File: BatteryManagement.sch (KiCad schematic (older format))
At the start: 1 part

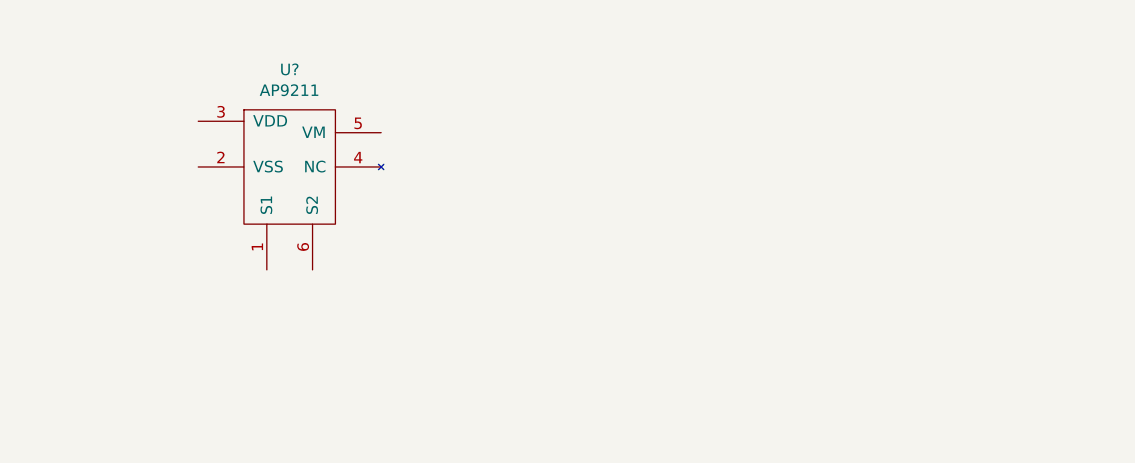
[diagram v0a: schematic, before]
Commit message: Battery work, need to get on to connectors.
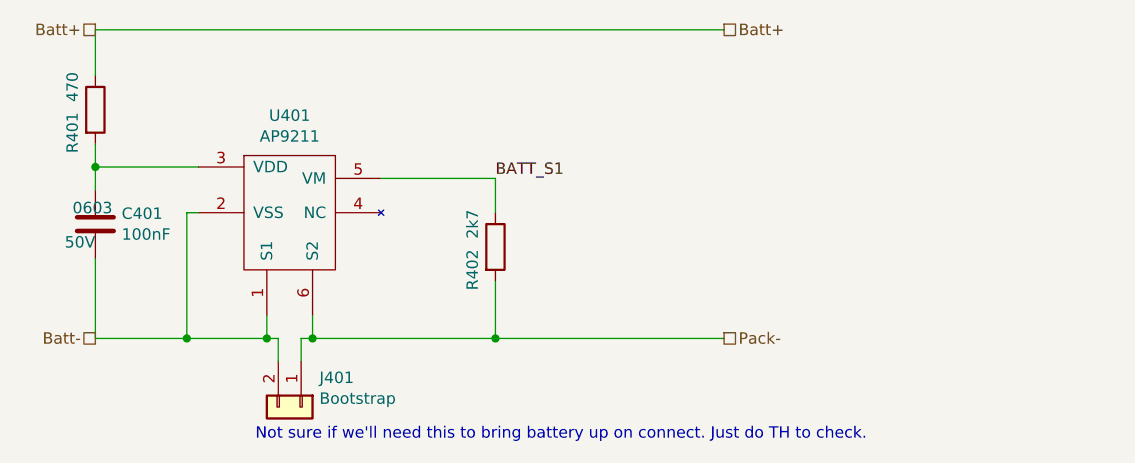
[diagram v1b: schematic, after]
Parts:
- added C401: 100nF, Capacitors_SMD:C_0603, symbol Device:C
- added J401: Bootstrap, Pin_Headers:Pin_Header_Straight_1x02_Pitch2.54mm, symbol Connector_Generic:Conn_01x02
- added R401: 470, Resistor_SMD:R_0603_1608Metric_Pad1.05x0.95mm_HandSolder, symbol Device:R
- added R402: 2k7, Resistor_SMD:R_0603_1608Metric_Pad1.05x0.95mm_HandSolder, symbol Device:R
- gave numbers to parts that had none: 1
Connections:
- net Batt-: now reaches U401.1 (S1)
- net Batt-: now also U401.2 (VSS), C401.2, J401.2 (Pin_2)
- net at U401.3 (VDD): now also C401.1, R401.2
- net BATT_S1: now reaches U401.5 (VM)
- net BATT_S1: now also R402.1
- net Pack-: now reaches U401.6 (S2)
- net Pack-: now also J401.1 (Pin_1), R402.2
- new net Batt+: R401.1
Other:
- note added: "Not sure if we'll need this to bring battery up on connect. Just do TH to check."
- moved on the sheet: U401
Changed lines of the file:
@@
 L dingo-hat:AP9211 U?
 U 1 1 5DC173E3
-P 5550 2800
+P 5550 3000
 AR Path="/5DA95EB0/5DAAD200/5DC173E3" Ref="U?"  Part="1"
-AR Path="/5DC297AB/5DC173E3" Ref="U?"  Part="1"
-F 0 "U?" H 5550 3225 50  0000 C CNN
-F 1 "AP9211" H 5550 3134 50  0000 C CNN
-F 2 "" H 5550 2650 50  0001 C CNN
-F 3 "https://www.diodes.com/assets/Datasheets/AP9211.pdf" H 5550 2650 50  0001 C CNN
-	1    5550 2800
+AR Path="/5DC297AB/5DC173E3" Ref="U401"  Part="1"
+F 0 "U401" H 5550 3425 50  0000 C CNN
+F 1 "AP9211" H 5550 3334 50  0000 C CNN
+F 2 "" H 5550 2850 50  0001 C CNN
+F 3 "https://www.diodes.com/assets/Datasheets/AP9211.pdf" H 5550 2850 50  0001 C CNN
+	1    5550 3000
 	1    0    0    -1
 $EndComp
+$Comp
+L Device:C C?
+U 1 1 5DD0667E
+P 4700 3050
+AR Path="/5DD0667E" Ref="C?"  Part="1"
+AR Path="/5DA95EB0/5DD0667E" Ref="C?"  Part="1"
+AR Path="/5DC297AB/5DD0667E" Ref="C401"  Part="1"
+F 0 "C401" H 4815 3096 50  0000 L CNN
+F 1 "100nF" H 4815 3005 50  0000 L CNN
+F 2 "Capacitors_SMD:C_0603" H 4738 2900 50  0001 C CNN
+F 3 "~" H 4700 3050 50  0001 C CNN
+F 4 "0603" H 4600 3150 50  0000 L TNN "Package"
+F 5 "CAP CER 0.1UF 50V X7R 0603" H 4700 3050 50  0001 C CNN "Description"
+F 6 "50V" H 4700 3000 50  0000 R TNN "Voltage Rating"
+F 7 "https://www.digikey.com/product-detail/en/samsung-electro-mechanics/CL10B104KB8NNNC/1276-1000-1-ND/3889086" H 4700 3050 50  0001 C CNN "Link"
+F 8 "Digi-Key" H 4700 3050 50  0001 C CNN "Supplier 1"
+F 9 "1276-1000-1-ND" H 4700 3050 50  0001 C CNN "Supplier Part Number 1"
+F 10 "0.15000" H 4700 3050 50  0001 C CNN "Unit Cost A$"
+	1    4700 3050
+	1    0    0    -1
+$EndComp
+$Comp
+L Device:R R?
+U 1 1 5DE42ED8
+P 6450 3150
+AR Path="/5DE42ED8" Ref="R?"  Part="1"
+AR Path="/5DC297AB/5DE42ED8" Ref="R402"  Part="1"
+F 0 "R402" V 6350 3050 50  0000 C CNN
+F 1 "2k7" V 6350 3250 50  0000 C CNN
+F 2 "Resistor_SMD:R_0603_1608Metric_Pad1.05x0.95mm_HandSolder" V 6380 3150 50  0001 C CNN
+F 3 "~" H 6450 3150 50  0001 C CNN
+F 4 "0603" H 5150 -2900 50  0001 C CNN "Package"
+	1    6450 3150
+	1    0    0    -1
+$EndComp
+Wire Wire Line
+	7450 3550 6450 3550
+Wire Wire Line
+	6450 3000 6450 2850
+Wire Wire Line
+	6450 2850 5950 2850
+Wire Wire Line
+	4700 2200 4700 2400
+Wire Wire Line
+	4700 2700 4700 2800
+Wire Wire Line
+	5450 3450 5450 3550
+Wire Wire Line
+	5450 3550 5100 3550
+Wire Wire Line
+	4700 3550 4700 3200
+Wire Wire Line
+	4700 2900 4700 2800
+Connection ~ 4700 2800
+Wire Wire Line
+	5150 3000 5100 3000
+Wire Wire Line
+	5100 3000 5100 3550
+Wire Wire Line
+	4700 3550 5100 3550
+Connection ~ 5100 3550
+Wire Wire Line
+	4700 2800 5150 2800
+Wire Wire Line
+	5650 3450 5650 3550
+Wire Wire Line
+	5650 3550 6450 3550
+Connection ~ 6450 3550
+Wire Wire Line
+	6450 3550 6450 3300
+Text HLabel 4700 2200 0    50   UnSpc ~ 0
+Batt+
+Text HLabel 7450 3550 2    50   UnSpc ~ 0
+Pack-
+Text HLabel 4700 3550 0    50   UnSpc ~ 0
+Batt-
+Wire Wire Line
+	4700 2200 7450 2200
+Text HLabel 7450 2200 2    50   UnSpc ~ 0
+Batt+
+$Comp
+L Device:R R?
+U 1 1 5DE426CE
+P 4700 2550
+AR Path="/5DE426CE" Ref="R?"  Part="1"
+AR Path="/5DC297AB/5DE426CE" Ref="R401"  Part="1"
+F 0 "R401" V 4600 2450 50  0000 C CNN
+F 1 "470" V 4600 2650 50  0000 C CNN
+F 2 "Resistor_SMD:R_0603_1608Metric_Pad1.05x0.95mm_HandSolder" V 4630 2550 50  0001 C CNN
+F 3 "~" H 4700 2550 50  0001 C CNN
+F 4 "0603" H 3400 -3500 50  0001 C CNN "Package"
+	1    4700 2550
+	1    0    0    -1
+$EndComp
+$Comp
+L Connector_Generic:Conn_01x02 J401
+U 1 1 5DE79FB0
+P 5600 3850
+F 0 "J401" V 5472 3930 50  0000 L CNN
+F 1 "Bootstrap" V 5563 3930 50  0000 L CNN
+F 2 "Pin_Headers:Pin_Header_Straight_1x02_Pitch2.54mm" H 5600 3850 50  0001 C CNN
+F 3 "~" H 5600 3850 50  0001 C CNN
+	1    5600 3850
+	0    1    1    0
+$EndComp
+Text Notes 5400 4000 0    50   ~ 0
+Not sure if we'll need this to bring battery up on connect. Just do TH to check.
+Wire Wire Line
+	5500 3650 5500 3550
+Wire Wire Line
+	5500 3550 5450 3550
+Connection ~ 5450 3550
+Wire Wire Line
+	5650 3550 5600 3550
+Wire Wire Line
+	5600 3550 5600 3650
+Connection ~ 5650 3550
+Text Label 6450 2850 0    50   ~ 0
+BATT_S1
 $EndSCHEMATC
